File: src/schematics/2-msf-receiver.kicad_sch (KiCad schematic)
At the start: 75 parts, among them U201 TPS7A2040PDQNR, U202 TPS7A2036PDBVR, U203 MCP6499, U204 MCP6499, U205 74HC595BQ

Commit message: Started to lay out the PCB.
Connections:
- net GND_PWRIN renamed GND

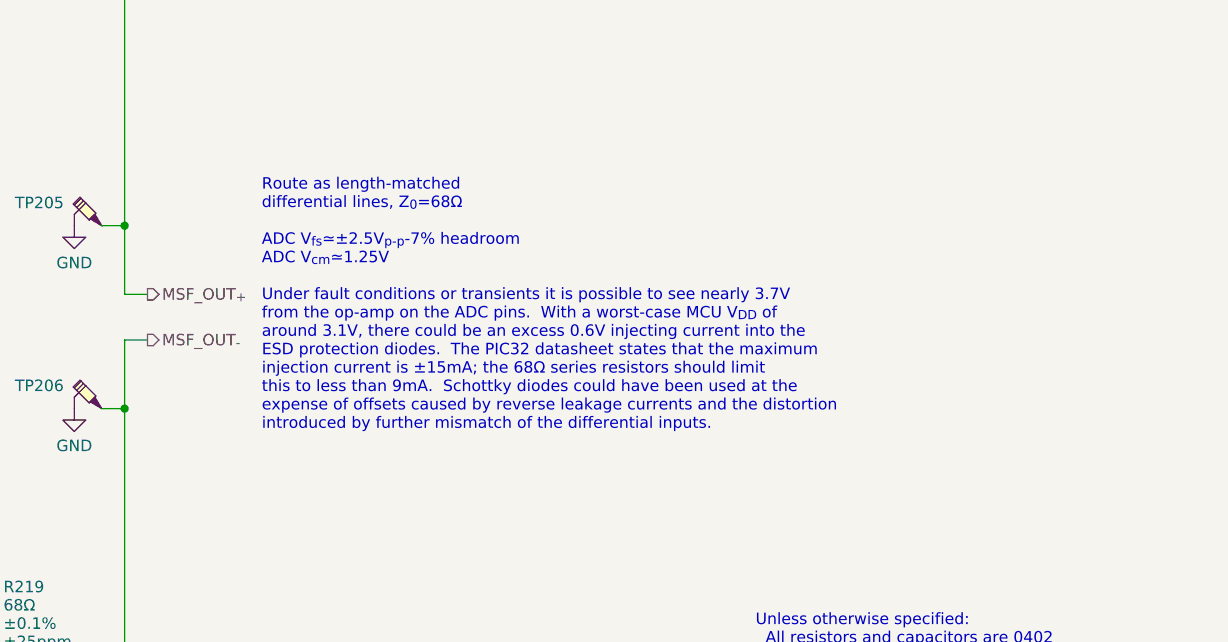
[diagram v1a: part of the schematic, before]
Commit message: PCB routing.
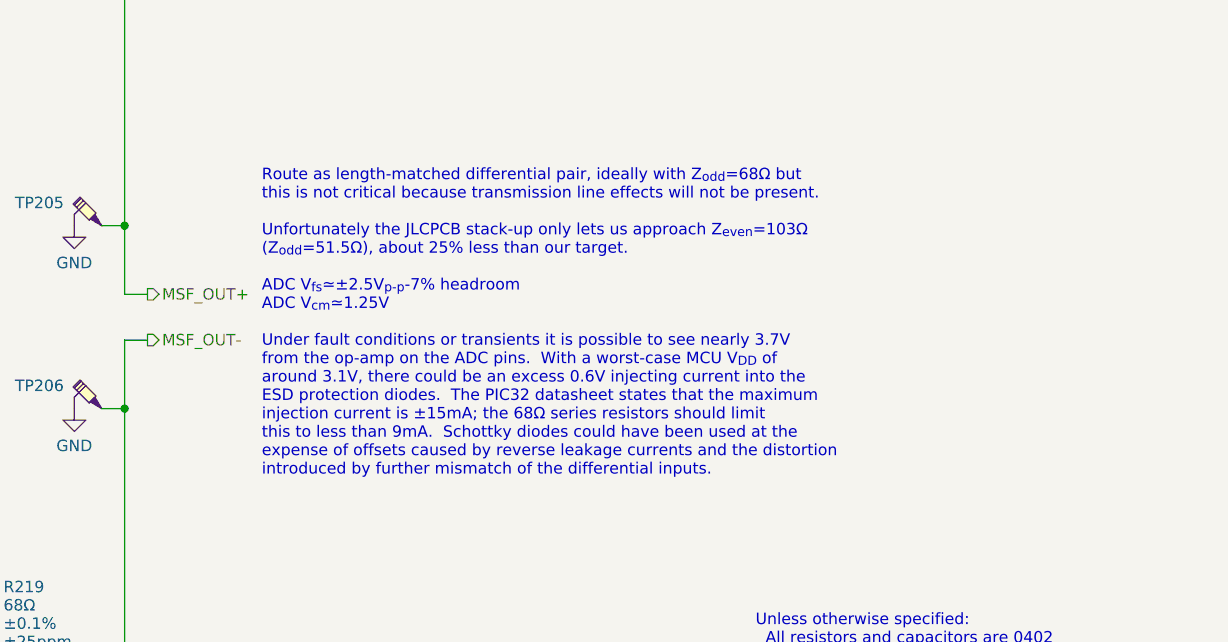
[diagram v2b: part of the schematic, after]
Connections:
- net MSF_OUT_{+} renamed MSF_OUT+
- net MSF_OUT_{-} renamed MSF_OUT-
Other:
- note added: "Route as length-matched differential pair, ideally with Z_{odd}=68Ω but this is not critical because transmission line effects will not be present. Unfortunately the JLCPCB stack-up only lets us approach Z_{even}=103Ω (Z_{odd}=51.5Ω), about 25% less than our target. ADC V_{fs}≃±2.5V_{p-p}-7% headroom ADC V_{cm}≃1.25V Under fault conditions or transients it is possible to see nearly 3.7V from the 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"
- note removed: "Route as length-matched differential lines, Z_{0}=68Ω ADC V_{fs}≃±2.5V_{p-p}-7% headroom ADC V_{cm}≃1.25V Under fault conditions or transients it is possible to see nearly 3.7V from the op-amp on the ADC pins. With a worst-case MCU V_{DD} of around 3.1V, there could be an excess 0.6V injecting current into the ESD protection diodes. The PIC32 datasheet states that the maximum injection current is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"
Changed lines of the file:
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@@
     (effects (font (size 1.27 1.27)) (justify left bottom))
   )
-  (text "Route as length-matched\ndifferential lines, Z_{0}=68Ω\n\nADC V_{fs}≃±2.5V_{p-p}-7% headroom\nADC V_{cm}≃1.25V\n\nUnder fault conditions or transients it is possible to see nearly 3.7V\nfrom the op-amp on the ADC pins.  With a worst-case MCU V_{DD} of\naround 3.1V, there could be an excess 0.6V injecting current into the\nESD protection diodes.  The PIC32 datasheet states that the maximum\ninjection current is ±15mA; the 68Ω series resistors should limit\nthis to less than 9mA.  Schottky diodes could have been used at the\nexpense of offsets caused by reverse leakage currents and the distortion\nintroduced by further mismatch of the differential inputs."
-    (at 246.38 233.68 0)
+  (text "Route as length-matched differential pair, ideally with Z_{odd}=68Ω but\nthis is not critical because transmission line effects will not be present.\n\nUnfortunately the JLCPCB stack-up only lets us approach Z_{even}=103Ω\n(Z_{odd}=51.5Ω), about 25% less than our target.\n\nADC V_{fs}≃±2.5V_{p-p}-7% headroom\nADC V_{cm}≃1.25V\n\nUnder fault conditions or transients it is possible to see nearly 3.7V\nfrom the op-amp on the ADC pins.  With a worst-case MCU V_{DD} of\naround 3.1V, there could be an excess 0.6V injecting current into the\nESD protection diodes.  The PIC32 datasheet states that the maximum\ninjection current is ±15mA; the 68Ω series resistors should limit\nthis to less than 9mA.  Schottky diodes could have been used at the\nexpense of offsets caused by reverse leakage currents and the distortion\nintroduced by further mismatch of the differential inputs."
+    (at 246.38 238.76 0)
     (effects (font (size 1.27 1.27)) (justify left bottom))
   )
@@
     (effects (font (size 1.27 1.27)) (justify right))
   )
-  (hierarchical_label "MSF_OUT_{+}" (shape output) (at 233.68 218.44 0) (fields_autoplaced)
+  (hierarchical_label "MSF_OUT+" (shape output) (at 233.68 218.44 0) (fields_autoplaced)
     (effects (font (size 1.27 1.27)) (justify left))
   )
@@
     (effects (font (size 1.27 1.27)) (justify left))
   )
-  (hierarchical_label "MSF_OUT_{-}" (shape output) (at 233.68 223.52 0) (fields_autoplaced)
+  (hierarchical_label "MSF_OUT-" (shape output) (at 233.68 223.52 0) (fields_autoplaced)
     (effects (font (size 1.27 1.27)) (justify left))
   )

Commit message: PCB routing.
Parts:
- TP203, TP204: footprint restall-generic-test:testpoint-SP3050A-with-short-gnd -> restall-generic-test:th-testpoint-0.5mm-with-short-gnd
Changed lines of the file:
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@@
       (effects (font (size 1.27 1.27)) (justify right) hide)
     )
-    (property "Footprint" "restall-generic-test:testpoint-SP3050A-with-short-gnd" (at 127 92.71 0)
+    (property "Footprint" "restall-generic-test:th-testpoint-0.5mm-with-short-gnd" (at 127 92.71 0)
       (effects (font (size 1.27 1.27)) (justify right) hide)
     )
@@
       (effects (font (size 1.27 1.27)) (justify right) hide)
     )
-    (property "Footprint" "restall-generic-test:testpoint-SP3050A-with-short-gnd" (at 337.82 92.71 0)
-      (effects (font (size 1.27 1.27)) (justify right) hide)
-    )
+    (property "Footprint" "restall-generic-test:th-testpoint-0.5mm-with-short-gnd" (at 337.82 92.71 0)
+      (effects (font (size 1.27 1.27)) (justify right) hide)
+    )
